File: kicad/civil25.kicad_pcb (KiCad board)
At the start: 2 copper layers, 8 parts, among them U1 8088_Min_Mode, U2 SST39SF020, U3 AS6C4008-55PCN, U4 74HC245, U5 74HC373, U6 74HC373, U7 74HCT238, U8 74HC00

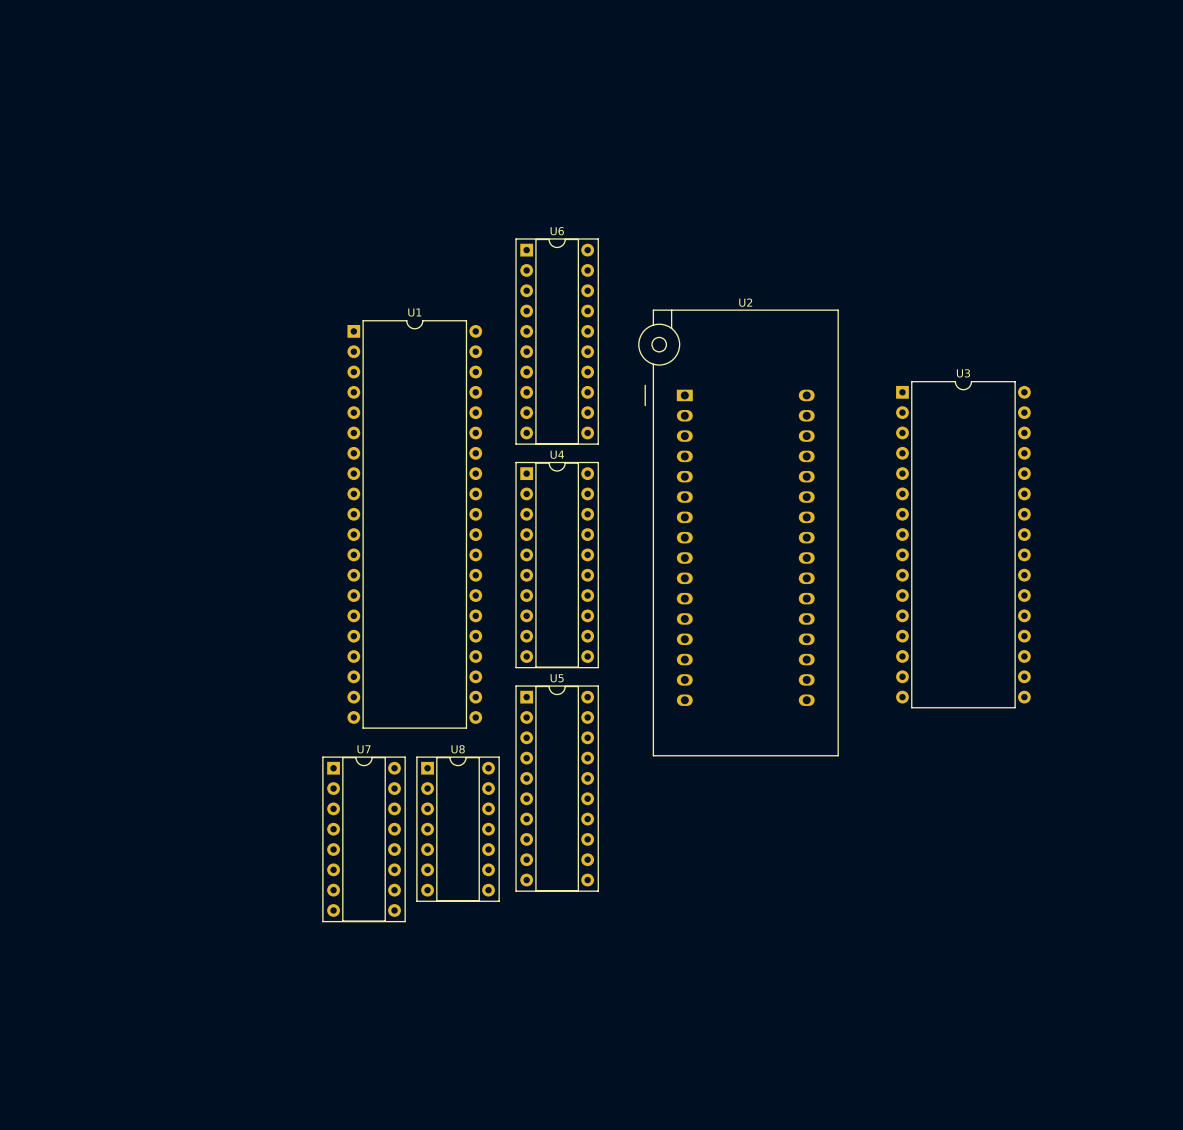
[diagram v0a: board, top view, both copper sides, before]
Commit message: update PCB
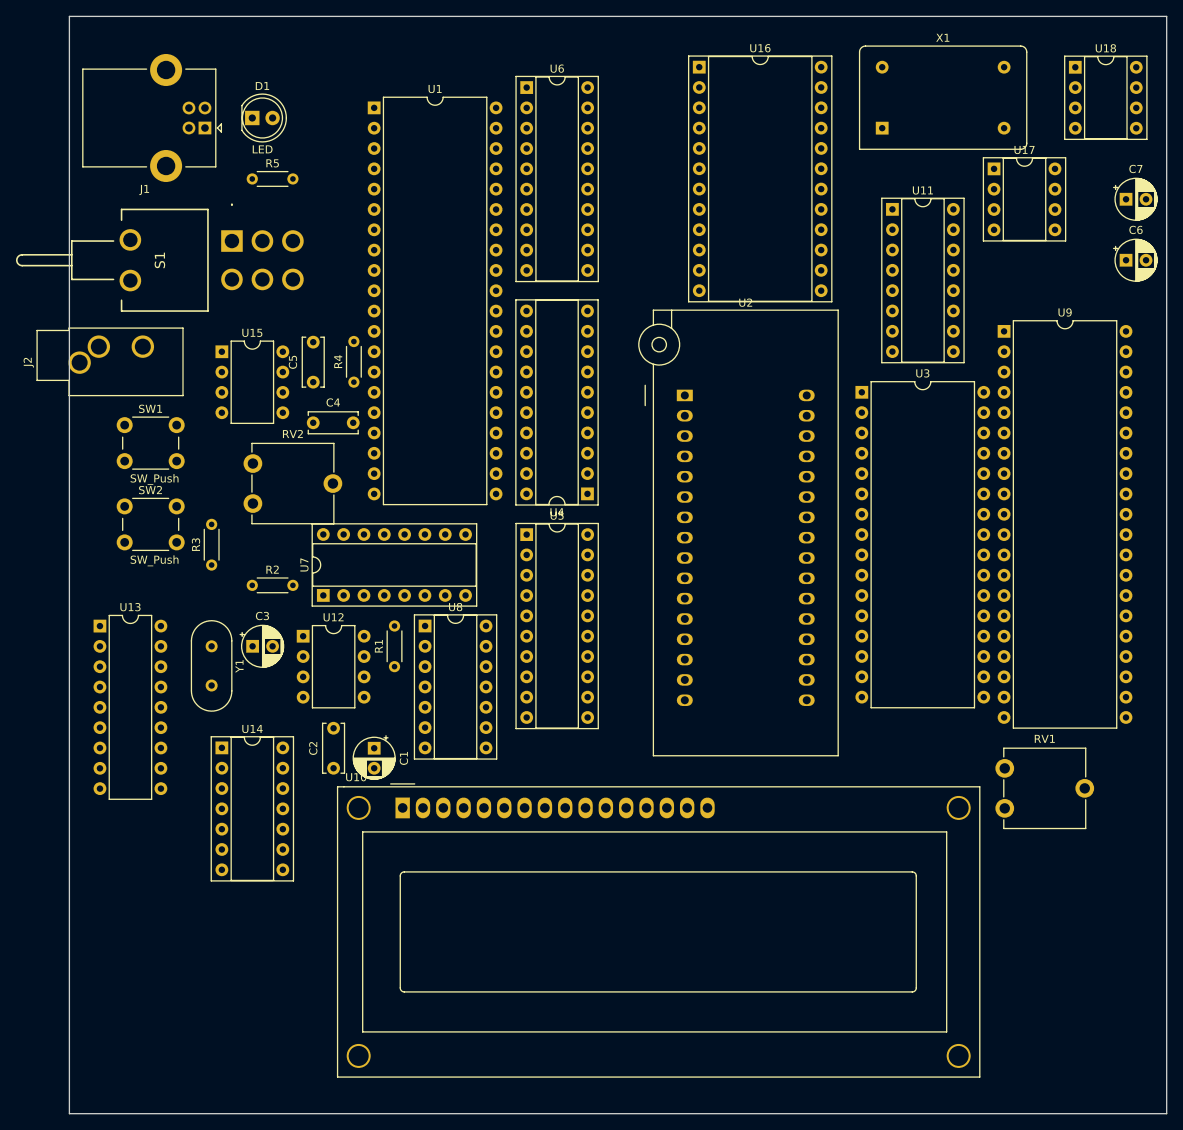
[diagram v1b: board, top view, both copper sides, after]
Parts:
- added C1: 1uF, Capacitor_THT:CP_Radial_D5.0mm_P2.50mm, F.Cu at (99.1, 119.4)
- added C2: 100nF, Capacitor_THT:C_Disc_D6.0mm_W2.5mm_P5.00mm, F.Cu at (94.0, 121.9)
- added C3: 4.7uF, Capacitor_THT:CP_Radial_D5.0mm_P2.50mm, F.Cu at (83.9, 106.7)
- added C4: 100nF, Capacitor_THT:C_Disc_D6.0mm_W2.5mm_P5.00mm, F.Cu at (91.4, 78.7)
- added C5: 100nF, Capacitor_THT:C_Disc_D6.0mm_W2.5mm_P5.00mm, F.Cu at (91.4, 73.7)
- added C6: 10uf, Capacitor_THT:CP_Radial_D5.0mm_P2.50mm, F.Cu at (193.0, 58.4)
- added C7: 1000uf, Capacitor_THT:CP_Radial_D5.0mm_P2.50mm, F.Cu at (193.0, 50.8)
- added D1: LED, LED_THT:LED_D5.0mm, F.Cu at (83.8, 40.6)
- added J1: USB_B, Connector_USB:USB_B_Lumberg_2411_02_Horizontal, F.Cu at (77.9, 41.9)
- added J2: AudioJack3, Connector_Audio:Jack_3.5mm_CUI_SJ1-3533NG_Horizontal_CircularHoles, F.Cu at (62.2, 71.2)
- added R1: 1k, Resistor_THT:R_Axial_DIN0204_L3.6mm_D1.6mm_P5.08mm_Horizontal, F.Cu at (101.6, 109.2)
- added R2: 10k, Resistor_THT:R_Axial_DIN0204_L3.6mm_D1.6mm_P5.08mm_Horizontal, F.Cu at (83.8, 99.1)
- added R3: 1k, Resistor_THT:R_Axial_DIN0204_L3.6mm_D1.6mm_P5.08mm_Horizontal, F.Cu at (78.7, 96.5)
- added R4: 1M, Resistor_THT:R_Axial_DIN0204_L3.6mm_D1.6mm_P5.08mm_Horizontal, F.Cu at (96.5, 73.7)
- added R5: 330, Resistor_THT:R_Axial_DIN0204_L3.6mm_D1.6mm_P5.08mm_Horizontal, F.Cu at (83.8, 48.3)
- added RV1: 10k, Potentiometer_THT:Potentiometer_ACP_CA9-V10_Vertical, F.Cu at (177.9, 126.9)
- added RV2: 1M, Potentiometer_THT:Potentiometer_ACP_CA9-V10_Vertical, F.Cu at (83.9, 88.8)
- added S1: M2024SA2G40, SamacSys_Parts:M2024SA2G40, F.Cu at (81.3, 56.0)
- added SW1: SW_Push, Button_Switch_THT:SW_PUSH_6mm_H4.3mm, F.Cu at (67.9, 79.0)
- added SW2: SW_Push, Button_Switch_THT:SW_PUSH_6mm_H4.3mm, F.Cu at (67.9, 89.2)
- added U10: LCD-016N002L, Display:WC1602A, F.Cu at (102.6, 126.9)
- added U11: 74LS138, Package_DIP:DIP-16_W7.62mm_Socket, F.Cu at (163.8, 52.1)
- added U12: LM555xN, Package_DIP:DIP-8_W7.62mm, F.Cu at (90.2, 105.4)
- added U13: 8284, Package_DIP:DIP-18_W7.62mm, F.Cu at (64.8, 104.2)
- added U14: 74LS10, Package_DIP:DIP-14_W7.62mm_Socket, F.Cu at (80.0, 119.4)
- added U15: LM555xN, Package_DIP:DIP-8_W7.62mm, F.Cu at (80.0, 69.9)
- added U16: YM3812, Package_DIP:DIP-24_W15.24mm_Socket, F.Cu at (139.7, 34.3)
- added U17: Y3014B, Package_DIP:DIP-8_W7.62mm_Socket, F.Cu at (176.5, 47.0)
- added U18: TL072, Package_DIP:DIP-8_W7.62mm_Socket, F.Cu at (186.7, 34.3)
- added U9: 82C55A, Package_DIP:DIP-40_W15.24mm, F.Cu at (177.8, 67.3)
- added X1: 3.579545MHz, Oscillator:Oscillator_DIP-14, F.Cu at (162.6, 41.9)
- added Y1: 15mHz, Crystal:Crystal_HC18-U_Vertical, F.Cu at (78.7, 106.7)
- U8: value 74HC00 -> 74HC14
- moved U1 28.1 mm to (99.1, 39.4)
- moved U7 21.6 mm to (92.7, 100.3), turned to 90 degrees
- moved U6 20.3 mm to (118.1, 36.8)
- moved U5 20.3 mm to (118.1, 92.7)
- moved U8 17.8 mm to (105.4, 104.1)
- moved U4 8.01 mm to (125.7, 87.6), turned to 180 degrees
- moved U3 5.08 mm to (160.0, 74.9)
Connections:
- net /A16/S3 renamed /S3
- net /A17/S4 renamed /S4
- net /A18/S5 renamed /S5
- net /A19/S6 renamed /S6
- net /D0 renamed D0
- net /D1 renamed D1
- net /D2 renamed D2
- net /D3 renamed D3
- net /D4 renamed D4
- net /D5 renamed D5
- net /D6 renamed D6
- net /D7 renamed D7
- net Net-(U1-Pad25) renamed /ALE
- net Net-(U1-Pad26) renamed /DEN
- net Net-(U1-Pad27) renamed /DT/R
- net Net-(U1-Pad28) renamed RD/
- net Net-(U1-Pad29) renamed WR
- net Net-(U1-Pad32) renamed IO/M/
- net Net-(U2-Pad24) renamed /MEMRD
- U1 pad 18: GND -> INTR
- U1 pad 19: unconnected-(U1-Pad19) -> CLK
- U1 pad 21: unconnected-(U1-Pad21) -> RESET
- U1 pad 22: unconnected-(U1-Pad22) -> READY
- U1 pad 34: GND -> unconnected-(U1-Pad34)
- U2 pad 12: /A0 -> A0
- U2 pad 22: Net-(U2-Pad22) -> /CE_ROM
- U3 pad 12: /A0 -> A0
- U3 pad 22: /A0 -> /A19
- U3 pad 24: GND -> /MEMWR
- U5 pad 2: /A0 -> A0
- U7 pad 13: GND -> /MEMWR
- U8 pad 1: /A18 -> RESET
- U8 pad 14: (no net) -> +5V
- U8 pad 2: /A19 -> Net-(U16-Pad3)
- U8 pad 3: Net-(U2-Pad22) -> (no net)
- U8 pad 7: (no net) -> GND
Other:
- board outline added: 137.2 x 137.2 mm
